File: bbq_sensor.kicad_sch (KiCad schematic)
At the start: 6 parts, among them J1 Battery_Conn, J2 USB-C_Conn, J3 Conn_01x06_Socket, U1 HT7333, U2 WEMOS_D1_mini

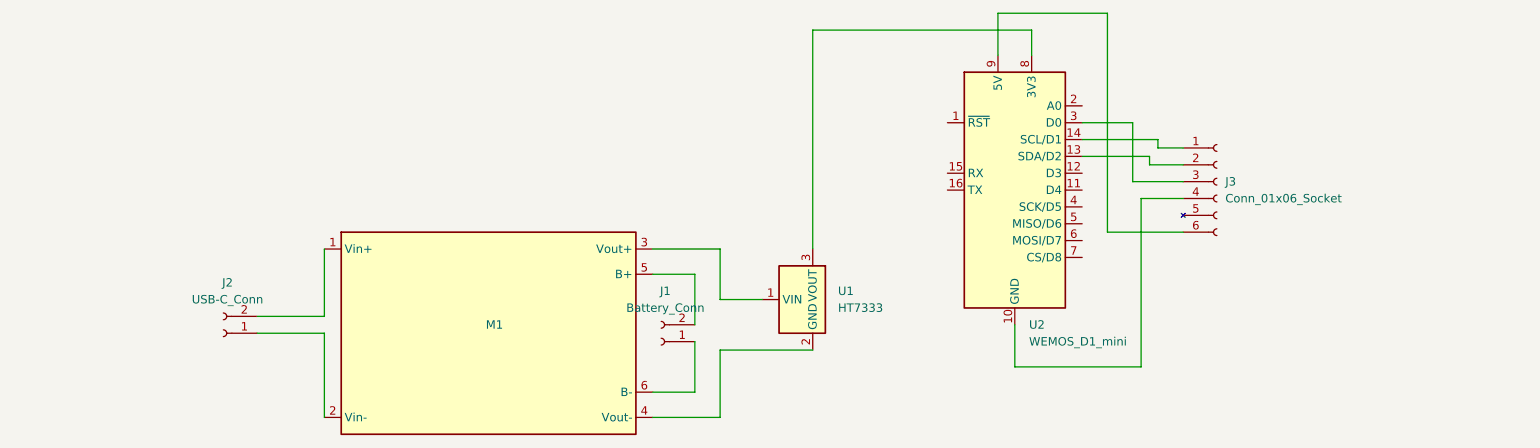
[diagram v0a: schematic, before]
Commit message: added caps
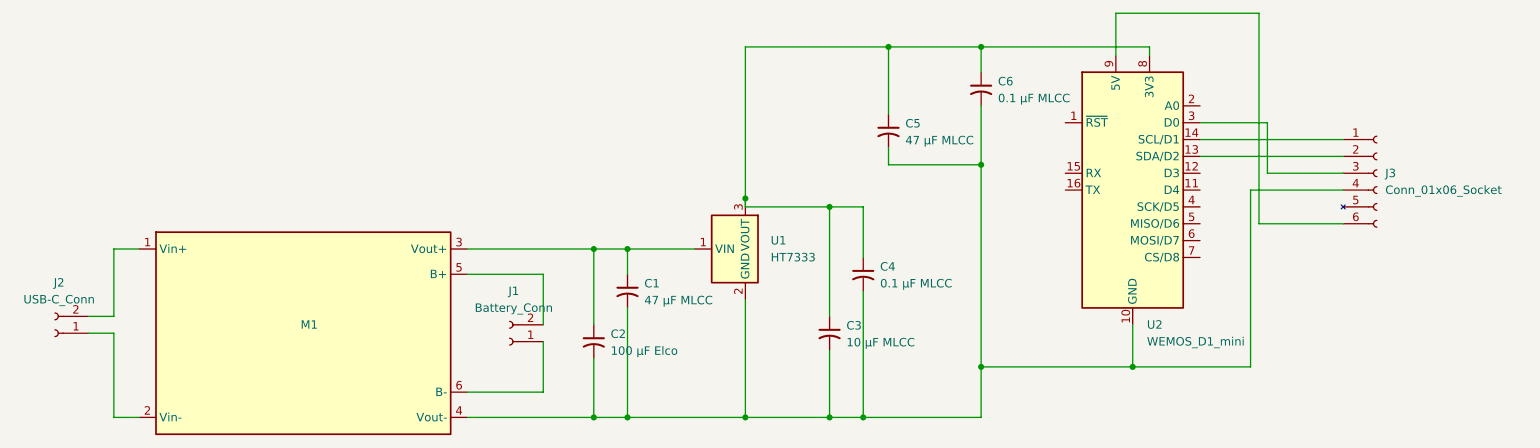
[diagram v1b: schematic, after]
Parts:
- added C1, C5: 47 µF MLCC, Capacitor_SMD:C_1206_3216Metric_Pad1.33x1.80mm_HandSolder, symbol Device:C_Small_US
- added C2: 100 µF Elco, Capacitor_SMD:C_1206_3216Metric_Pad1.33x1.80mm_HandSolder, symbol Device:C_Small_US
- added C3: 10 µF MLCC, Capacitor_SMD:C_1206_3216Metric_Pad1.33x1.80mm_HandSolder, symbol Device:C_Small_US
- added C4, C6: 0.1 µF MLCC, Capacitor_SMD:C_1206_3216Metric_Pad1.33x1.80mm_HandSolder, symbol Device:C_Small_US
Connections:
- net at J3.4 (GND), U2.10 (GND): now also M1.4 (Vout-), U1.2 (GND), C1.2, C2.2, C3.2, C4.2, C5.2, C6.2
- net at U1.3 (VOUT), U2.8 (3V3): now also C3.1, C4.1, C5.1, C6.1
- net at M1.3 (Vout+), U1.1 (VIN): now also C1.1, C2.1
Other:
- moved on the sheet: J1, J2, J3, M1, U1, U2
